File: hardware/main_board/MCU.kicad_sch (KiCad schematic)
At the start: 18 parts, among them J3 Conn_01x06_Pin, SW2 UP, U1 M0G3507QDGS32RQ1

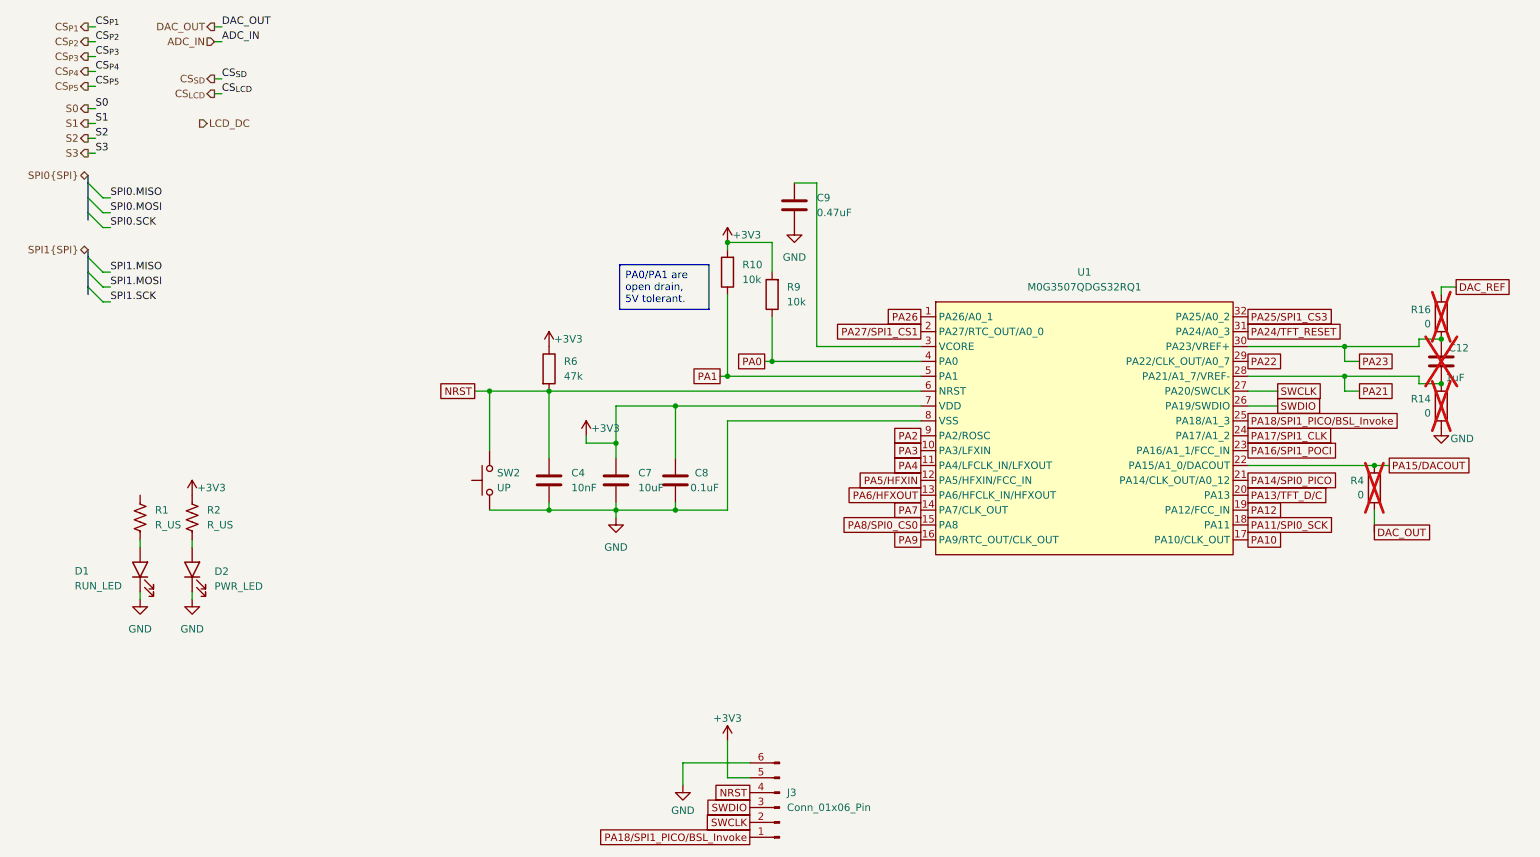
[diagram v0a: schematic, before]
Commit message: drew schematic
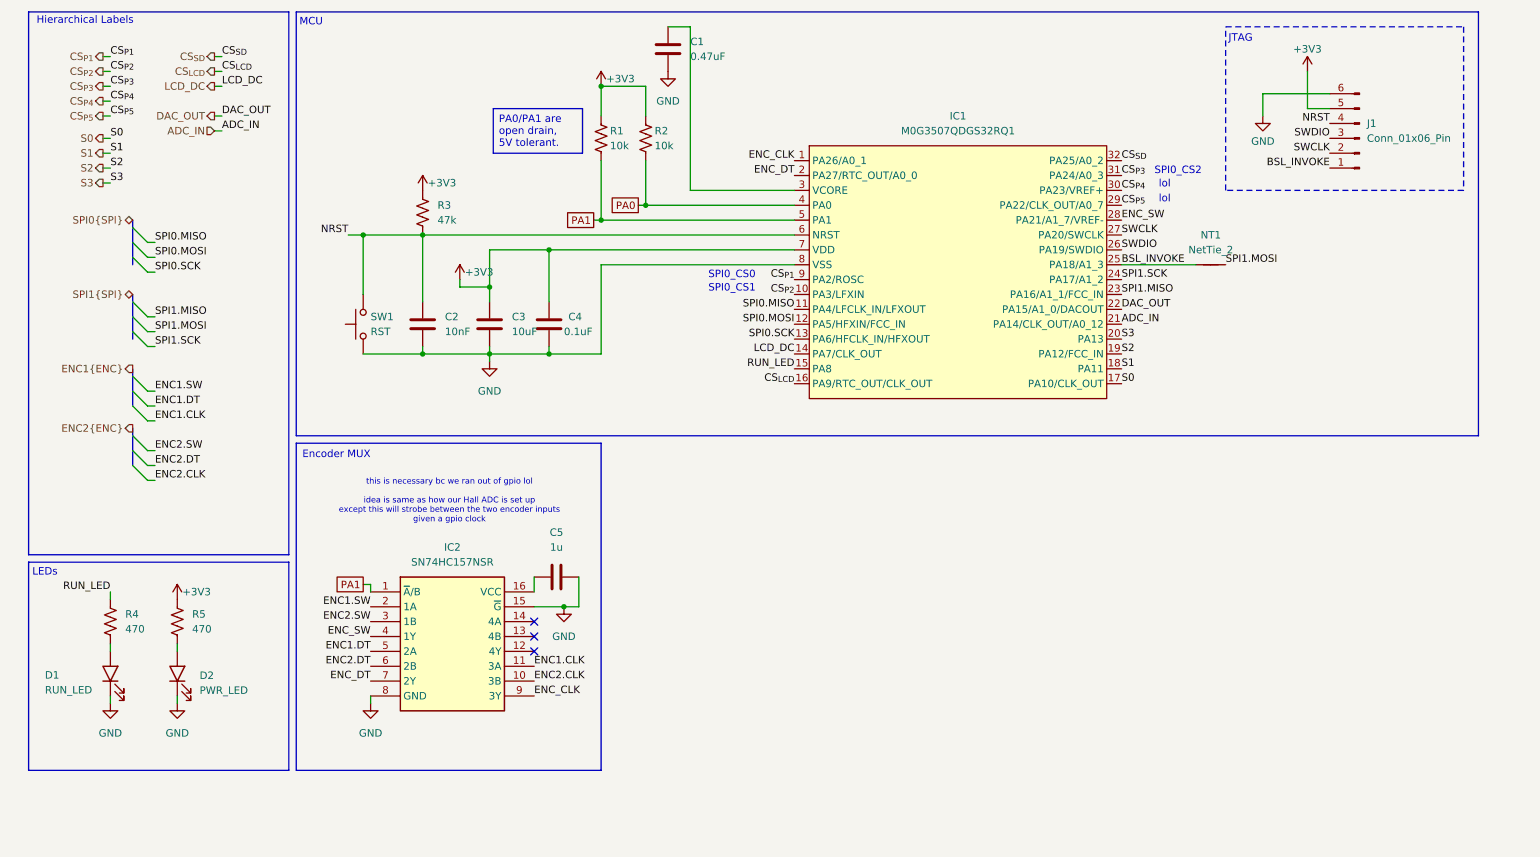
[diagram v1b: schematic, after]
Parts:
- removed C12: 1uF, Capacitor_THT:C_Disc_D6.0mm_W2.5mm_P5.00mm, symbol Device:C
- removed R14, R16, R4: 0, Jumper:SolderJumper-2_P1.3mm_Open_RoundedPad1.0x1.5mm, symbol Device:R
- added C5: 1u, Capacitor_SMD:C_0805_2012Metric, symbol ECE445L:C
- added IC2: SN74HC157NSR, SOIC127P780X200-16N, symbol SamacSys_Parts:SN74HC157NSR
- added NT1: NetTie_2, symbol Device:NetTie_2
- C1: renamed from C9; footprint Capacitor_THT:C_Disc_D6.0mm_W2.5mm_P5.00mm -> Capacitor_SMD:C_0805_2012Metric
- C2: renamed from C4; footprint Capacitor_THT:C_Disc_D6.0mm_W2.5mm_P5.00mm -> Capacitor_SMD:C_0805_2012Metric
- C3: renamed from C7; footprint Capacitor_THT:C_Disc_D6.0mm_W2.5mm_P5.00mm -> Capacitor_SMD:C_0805_2012Metric
- C4: renamed from C8; footprint Capacitor_THT:C_Disc_D6.0mm_W2.5mm_P5.00mm -> Capacitor_SMD:C_0805_2012Metric
- D1, D2: footprint ECE445L:LED_D5.0mm -> 445L:LED_D5.0mm
- R1: renamed from R10; footprint Resistor_THT:R_Axial_DIN0204_L3.6mm_D1.6mm_P7.62mm_Horizontal -> Resistor_SMD:R_0805_2012Metric; symbol Device:R -> Device:R_US
- R2: renamed from R9; footprint Resistor_THT:R_Axial_DIN0204_L3.6mm_D1.6mm_P7.62mm_Horizontal -> Resistor_SMD:R_0805_2012Metric; symbol Device:R -> Device:R_US
- R3: renamed from R6; footprint Resistor_THT:R_Axial_DIN0204_L3.6mm_D1.6mm_P7.62mm_Horizontal -> Resistor_SMD:R_0805_2012Metric; symbol Device:R -> Device:R_US
- R4: renamed from R1; value R_US -> 470; footprint (none) -> Resistor_SMD:R_0805_2012Metric
- R5: renamed from R2; value R_US -> 470; footprint (none) -> Resistor_SMD:R_0805_2012Metric
- SW1: renamed from SW2; value UP -> RST; footprint ECE445L:SW_PUSH_6mm -> 445L:SW_PUSH_6mm
- renumbered U1 to IC1, J3 to J1
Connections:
- net PA10 is gone; now on net S0: IC1.17 (PA10/CLK_OUT)
- net PA11/SPI0_SCK is gone; now on net S1: IC1.18 (PA11)
- net PA12 is gone; now on net S2: IC1.19 (PA12/FCC_IN)
- net PA13/TFT_D/C is gone; now on net S3: IC1.20 (PA13)
- net PA14/SPI0_PICO is gone; now on net ADC_IN: IC1.21 (PA14/CLK_OUT/A0_12)
- net PA15/DACOUT is gone; now on net DAC_OUT: IC1.22 (PA15/A1_0/DACOUT)
- net PA16/SPI1_POCI is gone; now on net SPI1.MISO: IC1.23 (PA16/A1_1/FCC_IN)
- net PA17/SPI1_CLK is gone; now on net SPI1.SCK: IC1.24 (PA17/A1_2)
- net PA2 is gone; now on net CS_{P1}: IC1.9 (PA2/ROSC)
- net PA22 is gone; now on net CS_{P5}: IC1.29 (PA22/CLK_OUT/A0_7)
- net PA23 is gone; now on net CS_{P4}: IC1.30 (PA23/VREF+)
- net PA24/TFT_RESET is gone; now on net CS_{P3}: IC1.31 (PA24/A0_3)
- net PA25/SPI1_CS3 is gone; now on net CS_{SD}: IC1.32 (PA25/A0_2)
- net PA3 is gone; now on net CS_{P2}: IC1.10 (PA3/LFXIN)
- net PA4 is gone; now on net SPI0.MISO: IC1.11 (PA4/LFCLK_IN/LFXOUT)
- net PA5/HFXIN is gone; now on net SPI0.MOSI: IC1.12 (PA5/HFXIN/FCC_IN)
- net PA6/HFXOUT is gone; now on net SPI0.SCK: IC1.13 (PA6/HFCLK_IN/HFXOUT)
- net PA7 is gone; now on net LCD_DC: IC1.14 (PA7/CLK_OUT)
- net PA8/SPI0_CS0 is gone; now on net RUN_LED: IC1.15 (PA8)
- net PA9 is gone; now on net CS_{LCD}: IC1.16 (PA9/RTC_OUT/CLK_OUT)
- net GND: now also C5.2, IC2.15 (~{G}), IC2.8 (GND)
- net PA1: now also IC2.1 (~{A}/B)
- net SPI1.MOSI: now also NT1.2
- net RUN_LED: now reaches R4.1
- net PA18/SPI1_PICO/BSL_Invoke renamed BSL_INVOKE
- net BSL_INVOKE: now also NT1.1
- net PA21 renamed ENC_SW
- net ENC_SW: now also IC2.4 (1Y)
- net PA26 renamed ENC_CLK
- net ENC_CLK: now also IC2.9 (3Y)
- net PA27/SPI1_CS1 renamed ENC_DT
- net ENC_DT: now also IC2.7 (2Y)
- new net: C5.1, IC2.16 (VCC)
- new net ENC1.CLK: IC2.11 (3A)
- new net ENC1.DT: IC2.5 (2A)
- new net ENC1.SW: IC2.2 (1A)
- new net ENC2.CLK: IC2.10 (3B)
- new net ENC2.DT: IC2.6 (2B)
- new net ENC2.SW: IC2.3 (1B)
- no-connect marks 0 -> 3
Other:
- note added: "Encoder MUX"
- note added: "Hierarchical Labels"
- note added: "JTAG"
- note added: "LEDs"
- note added: "MCU"
- note added: "SPI0_CS0"
- note added: "SPI0_CS1"
- note added: "SPI0_CS2"
- note added: "lol"
- note added: "this is necessary bc we ran out of gpio lol idea is same as how our Hall ADC is set up except this will strobe between the two encoder inputs given a gpio clock"
- moved on the sheet: C1, C2, C3, C4, D1, D2, IC1, J1, R4, R5, SW1
